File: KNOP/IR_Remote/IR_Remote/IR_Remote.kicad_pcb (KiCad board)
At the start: 2 copper layers, 153.5 x 53 mm, 51 parts, among them J1 Conn_01x01_Pin, J2 Conn_01x01_Pin, J3 Conn_01x02_Pin, J4 Conn_01x01_Pin, J5 Conn_01x01_Pin, J6 Conn_01x01_Pin, K1 Relay_SPDT, SW1 SW_Push, T1 BC327, T2 BC337, T3 BC547, T4 BC547

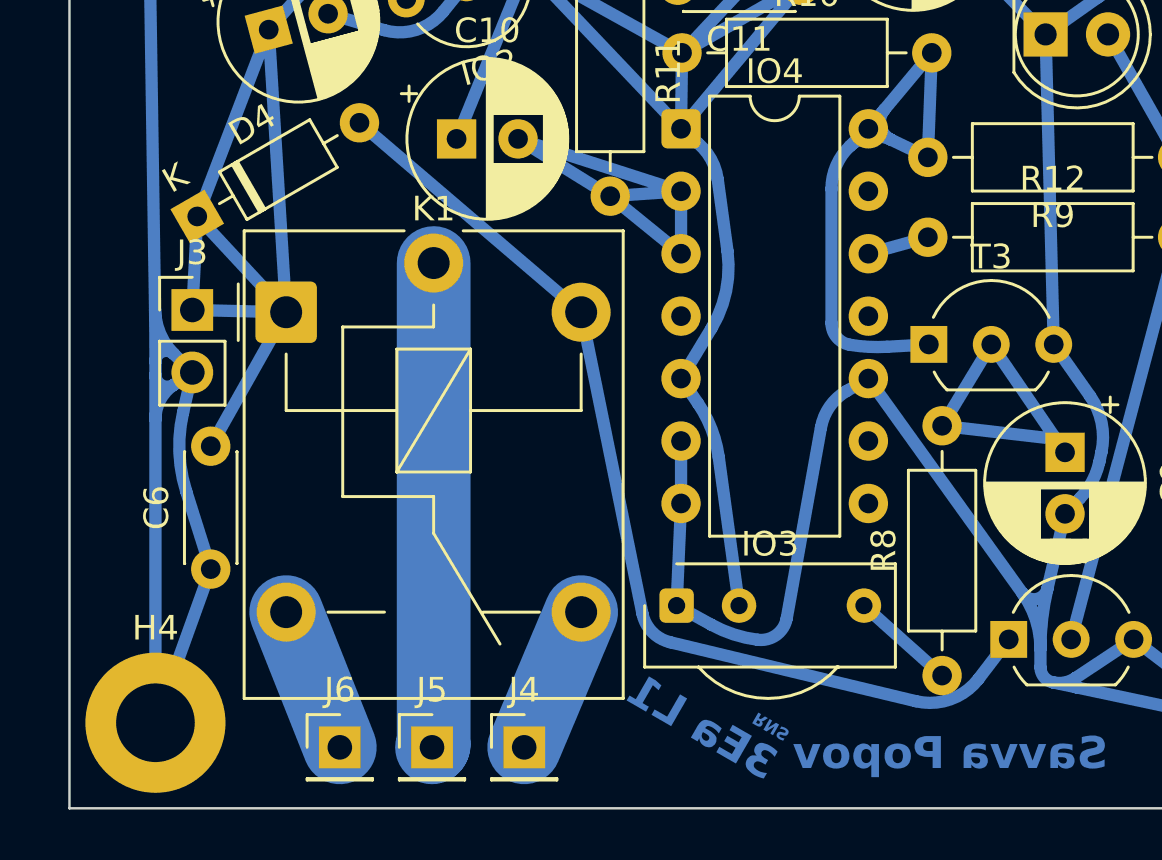
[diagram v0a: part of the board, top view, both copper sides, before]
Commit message: charlies sd
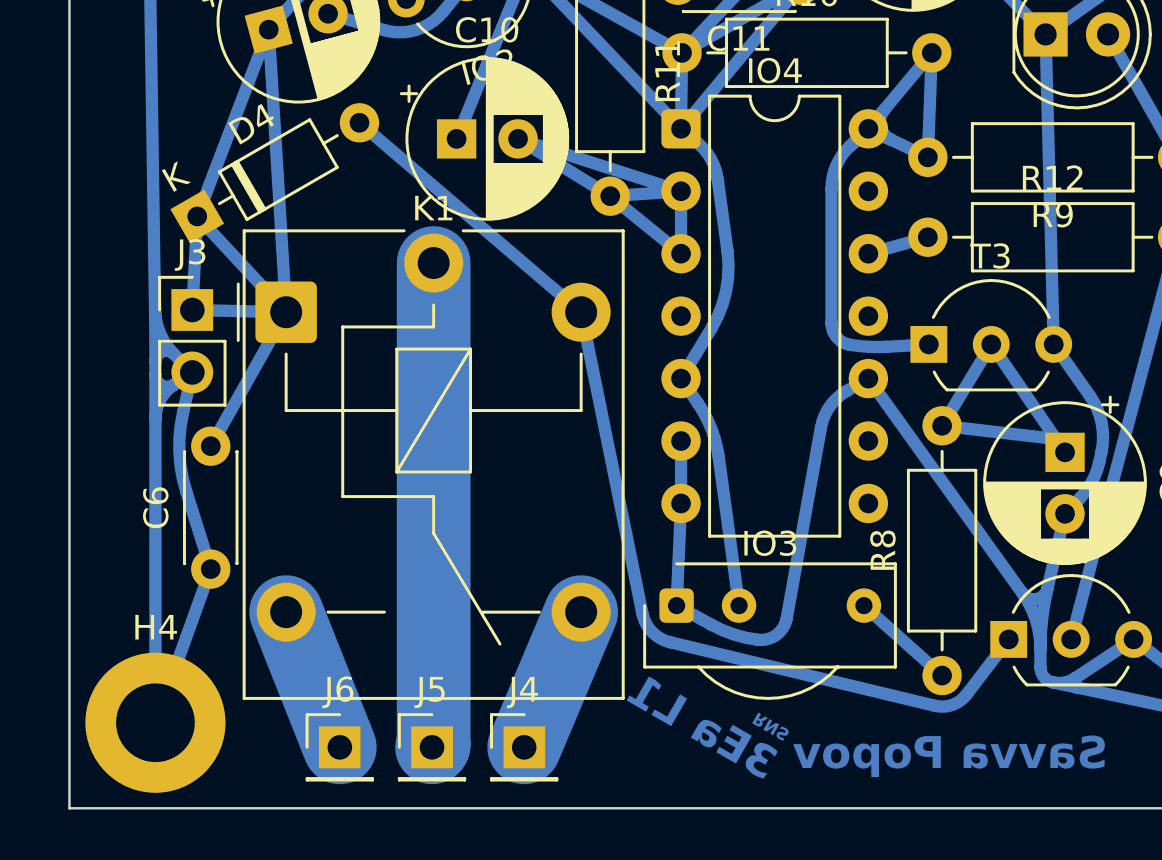
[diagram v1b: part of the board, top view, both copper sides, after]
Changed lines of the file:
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@@
 		(fp_line
 			(start 6.580001 0)
-			(end 5.929999 0)
+			(end 5.929999 0.000001)
 			(stroke
 				(width 0.12)
@@
 		)
 		(fp_text user "K"
-			(at 0 -1.799999 30)
+			(at 0.000001 -1.799999 30)
 			(layer "F.SilkS")
 			(effects
@@
 		)
 		(fp_text user "K"
-			(at 0 -1.799999 30)
+			(at 0.000001 -1.799999 30)
 			(layer "F.Fab")
 			(effects
@@
 		)
 		(fp_arc
-			(start 4.864182 1.122794)
+			(start 4.864181 1.122794)
 			(mid 4.633902 1.509327)
 			(end 4.340001 1.849999)
@@
 		)
 		(fp_arc
-			(start 2.54 -2.599999)
+			(start 2.54 -2.6)
 			(mid 3.93698 -2.192817)
 			(end 4.896402 -1.098806)
@@
 			(start 0.1836 -1.098807)
 			(mid 1.14302 -2.192817)
-			(end 2.54 -2.599999)
+			(end 2.54 -2.6)
 			(stroke
 				(width 0.12)
@@
 		)
 		(fp_line
-			(start 1.81 -3.181999)
+			(start 1.81 -3.181998)
 			(end 1.81 -1.04)
 			(stroke
@@
 		)
 		(fp_line
-			(start 3.050999 -2.69)
+			(start 3.050998 -2.69)
 			(end 3.051 -1.04)
 			(stroke
@@
 		(fp_line
 			(start 3.331 1.04)
-			(end 3.330999 2.484)
+			(end 3.330998 2.484)
 			(stroke
 				(width 0.12)
@@
 	(segment
 		(start 144.434894 100.724375)
-		(end 154.429377 103.12305)
+		(end 155.212156 103.310917)
 		(width 0.5)
 		(layer "B.Cu")
@@
 	)
 	(segment
-		(start 156.981167 102.216934)
+		(start 156.492163 102.856399)
 		(end 158.21 100.61)
 		(width 0.5)
@@
 	)
 	(arc
-		(start 156.981167 102.216934)
-		(mid 155.839668 103.048476)
-		(end 154.429377 103.12305)
+		(start 156.492163 102.856399)
+		(mid 155.919574 103.27351)
+		(end 155.212156 103.310917)
 		(width 0.5)
 		(layer "B.Cu")
